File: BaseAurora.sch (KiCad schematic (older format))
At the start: 13 parts

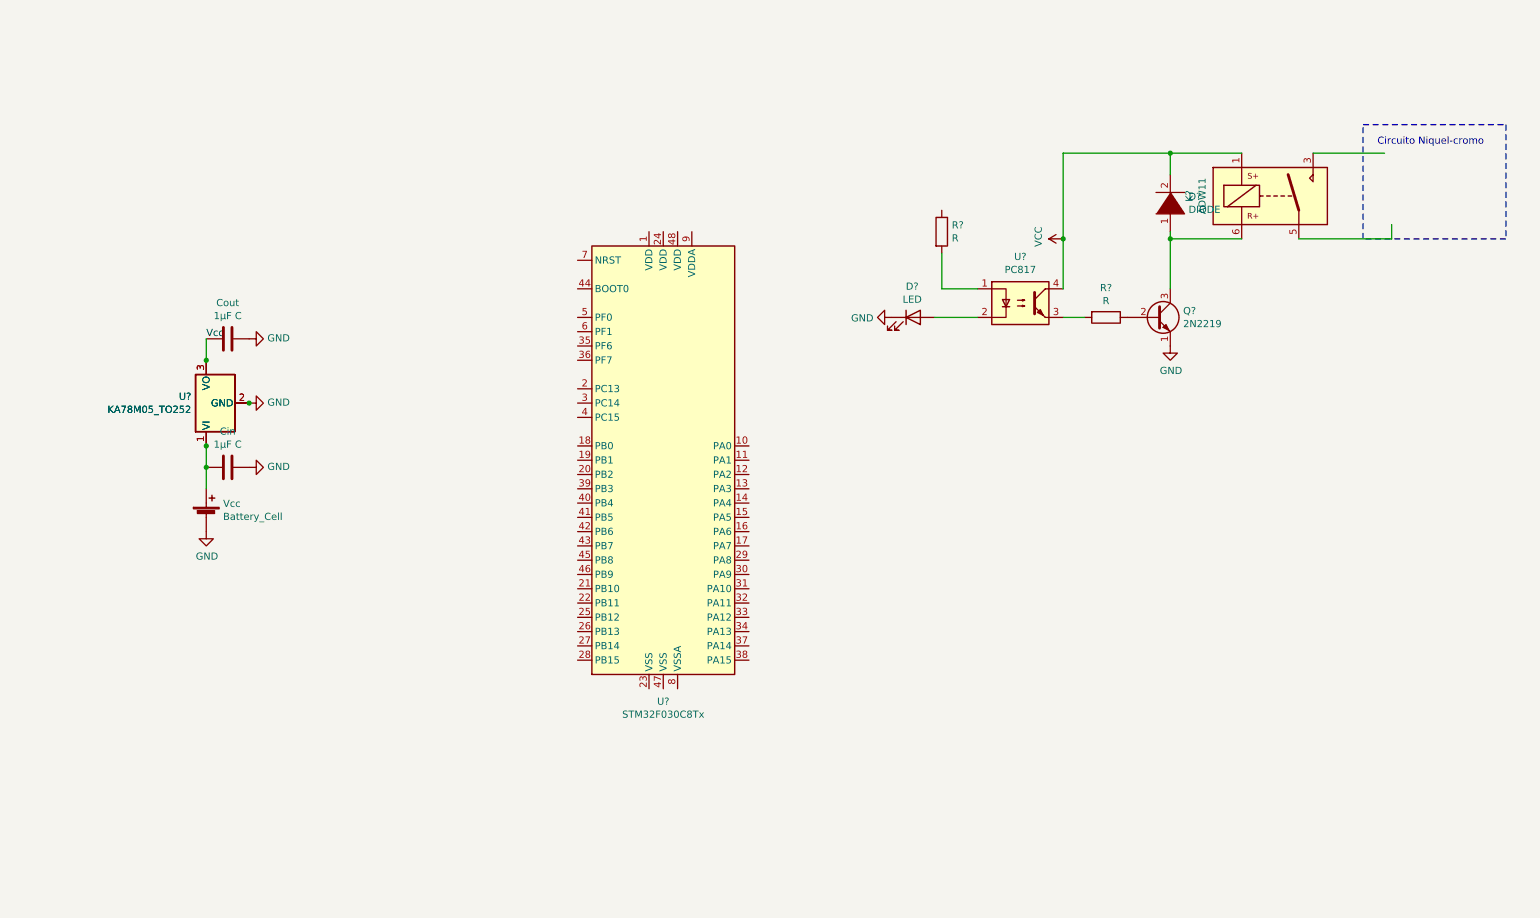
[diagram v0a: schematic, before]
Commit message: esquematico revisado
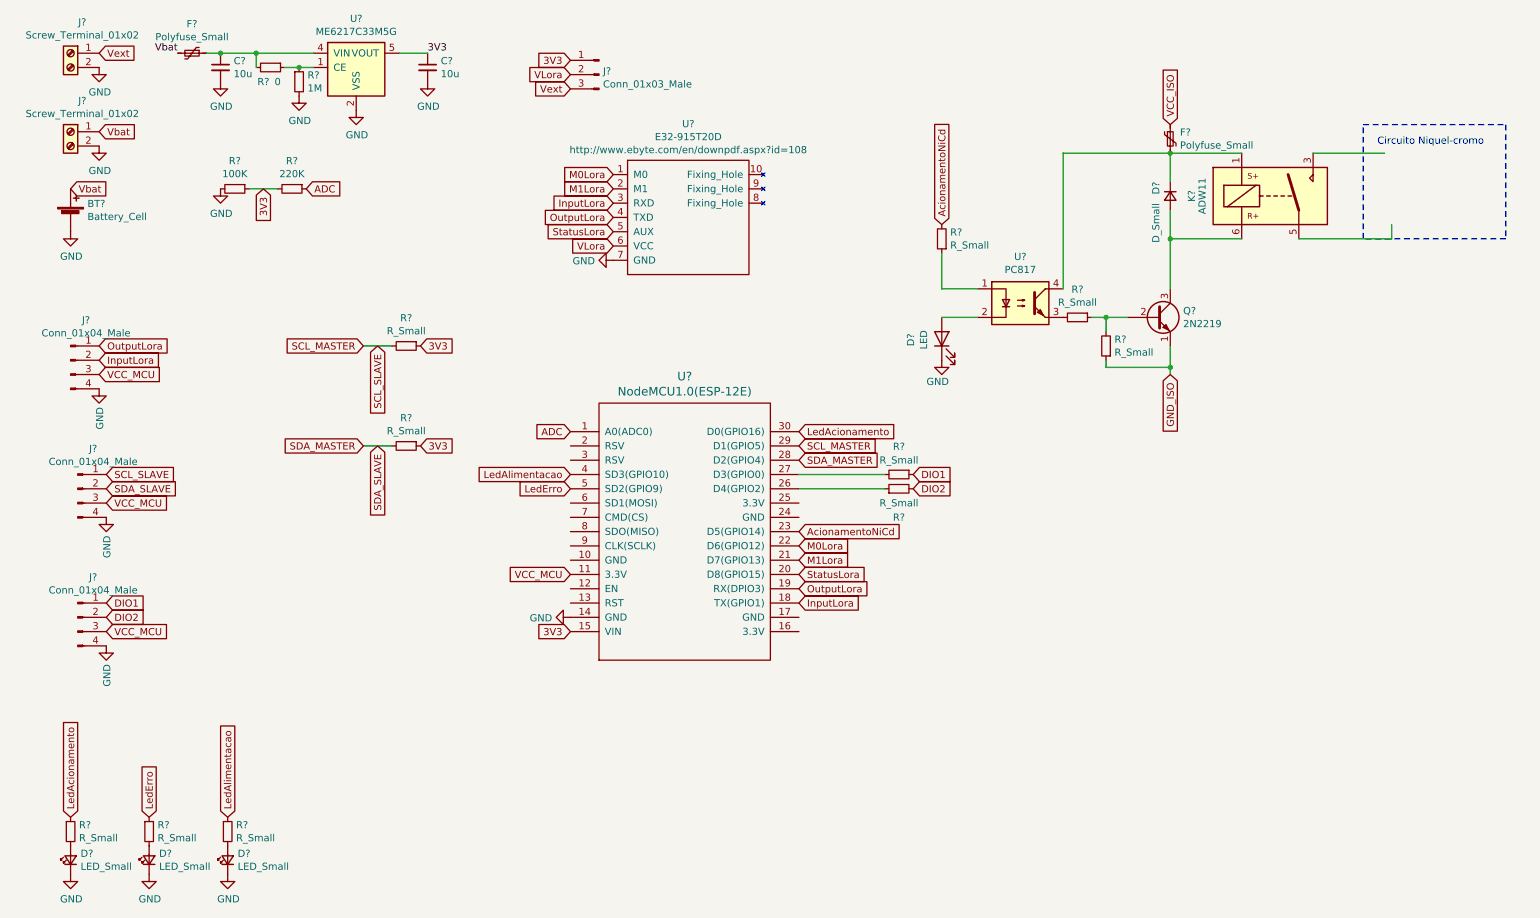
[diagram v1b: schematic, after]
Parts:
- removed Cin, Cout: 1μF C, symbol Device:C
- removed D?: DIODE, symbol pspice:DIODE
- removed R? (x2): R, symbol Device:R
- removed U?: STM32F030C8Tx, Package_QFP:LQFP-48_7x7mm_P0.5mm, symbol MCU_ST_STM32F0:STM32F030C8Tx
- removed U? (x2): KA78M05_TO252, Package_TO_SOT_SMD:TO-252-2, symbol Regulator_Linear:KA78M05_TO252
- removed Vcc: Battery_Cell, Battery:BatteryHolder_Keystone_2466_1xAAA, symbol Device:Battery_Cell
- added BT?: Battery_Cell, symbol Device:Battery_Cell
- added C? (x2): 10u, symbol Device:C_Small
- added D? (x3): LED_Small, symbol Device:LED_Small
- added D?: D_Small, symbol Device:D_Small
- added F? (x2): Polyfuse_Small, symbol Device:Polyfuse_Small
- added J? (x2): Screw_Terminal_01x02, symbol Connector:Screw_Terminal_01x02
- added J? (x3): Conn_01x04_Male, symbol Connector:Conn_01x04_Male
- added J?: Conn_01x03_Male, symbol Connector:Conn_01x03_Male
- added R? (x10): R_Small, symbol Device:R_Small
- added R?: 1M, symbol Device:R_Small
- added R?: 0, symbol Device:R_Small
- added R?: 100K, symbol Device:R_Small
- added R?: 220K, symbol Device:R_Small
- added U?: E32-915T20D, symbol LoRA:E32-915T20D
- added U?: ME6217C33M5G, symbol BaseAurora:ME6217C33M5G
- added U?: NodeMCU1.0(ESP-12E), symbol MCU_ESP82:NodeMCU1.0(ESP-12E)
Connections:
- net labels added: 3V3, ADC, AcionamentoNiCd, DIO1, DIO2, GND_ISO, InputLora, LedAcionamento, LedAlimentacao, LedErro, M0Lora, M1Lora, OutputLora, SCL_MASTER, SCL_SLAVE, SDA_MASTER, SDA_SLAVE, StatusLora, VCC_ISO, VCC_MCU, VLora, Vbat, Vext
- net labels removed: VCC, Vcc
- wire segments 18 -> 32
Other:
- moved on the sheet: D?
